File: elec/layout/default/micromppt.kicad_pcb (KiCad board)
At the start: 2 copper layers, 25.7 x 15.1 mm, 17 parts, among them U5 10µF ±20% 6.3V X5R

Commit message: fixed
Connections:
- C3 pad 1: hv-1 -> hv
- R1 pad 1: hv-1 -> hv
- R3 pad 1: hv -> hv-1
- R5 pad 2: hv-1 -> hv
- R6 pad 2: hv-1 -> hv
- U3 pad 1: hv -> hv-1
- U5 pad 1: hv -> hv-1
- U7 pad 1: hv-1 -> hv
- U8 pad 1: hv -> hv-1
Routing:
- net hv-1: track 18.5 -> 17.5 mm, vias 2 -> 0
- net hv: track 17.5 -> 18.5 mm, vias 0 -> 2
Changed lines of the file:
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@@
     (net 5 "cathode")
     (net 6 "VCTRL")
-    (net 7 "hv-1")
+    (net 7 "hv")
     (net 8 "gnd")
-    (net 9 "hv")
+    (net 9 "hv-1")
     (footprint "lib:SOT-23-6_L2.9-W1.6-P0.95-LS2.8-BR"
         (layer "F.Cu")
@@
             (size 0.57 0.54)
             (layers "F.Cu" "F.Mask" "F.Paste")
-            (net 7 "hv-1")
+            (net 7 "hv")
         )
         (pad "2" smd rect
@@
             (drill 0.900024)
             (layers "*.Cu" "*.Mask")
-            (net 9 "hv")
+            (net 9 "hv-1")
             (remove_unused_layers no)
         )
@@
             (size 0.8 0.9)
             (layers "F.Cu" "F.Mask" "F.Paste")
-            (net 9 "hv")
+            (net 9 "hv-1")
         )
         (pad "2" smd rect
@@
             (drill 0.900024)
             (layers "*.Cu" "*.Mask")
-            (net 7 "hv-1")
+            (net 7 "hv")
             (remove_unused_layers no)
         )
@@
             (size 0.57 0.54)
             (layers "F.Cu" "F.Mask" "F.Paste")
-            (net 7 "hv-1")
+            (net 7 "hv")
         )
         (embedded_fonts no)
@@
             (size 1.55 5.6)
             (layers "F.Cu" "F.Mask" "F.Paste")
-            (net 9 "hv")
+            (net 9 "hv-1")
             (pintype "stereo")
         )
@@
             (size 1.21 1.7)
             (layers "F.Cu" "F.Mask" "F.Paste")
-            (net 7 "hv-1")
+            (net 7 "hv")
         )
         (embedded_fonts no)
@@
             (size 0.8 0.9)
             (layers "F.Cu" "F.Mask" "F.Paste")
-            (net 7 "hv-1")
+            (net 7 "hv")
         )
         (pad "2" smd rect
@@
             (size 0.57 0.54)
             (layers "F.Cu" "F.Mask" "F.Paste")
-            (net 9 "hv")
+            (net 9 "hv-1")
         )
         (pad "2" smd rect

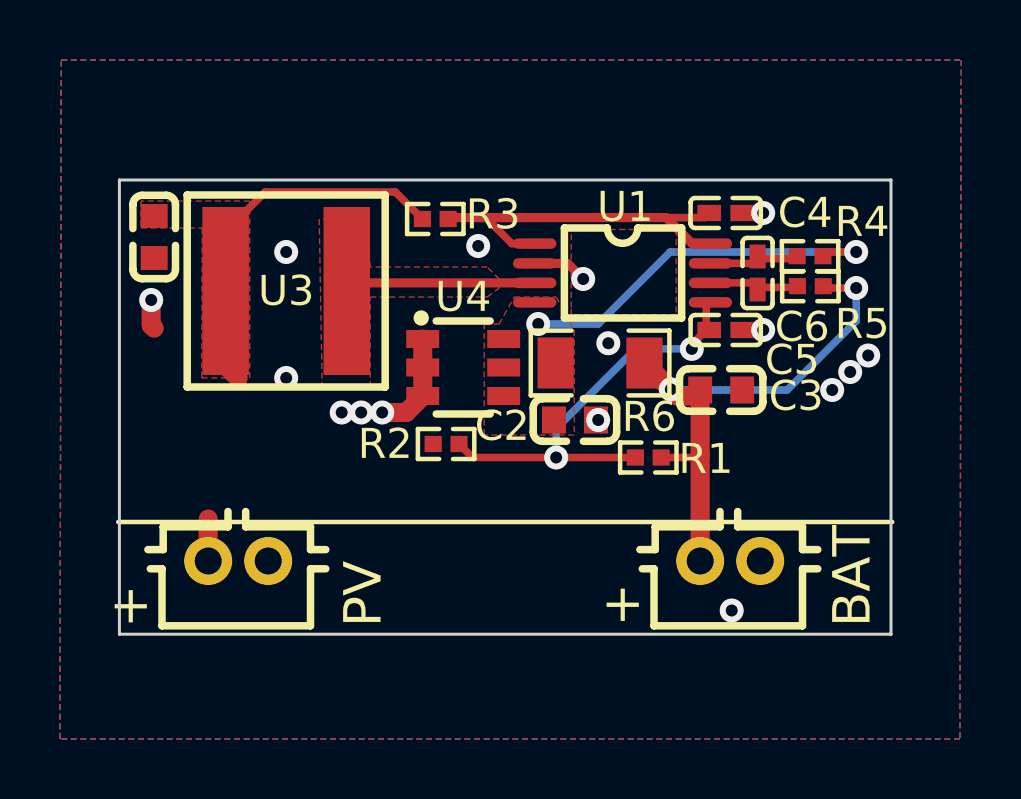
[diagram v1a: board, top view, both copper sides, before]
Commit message: ready for publishing on the ato repo
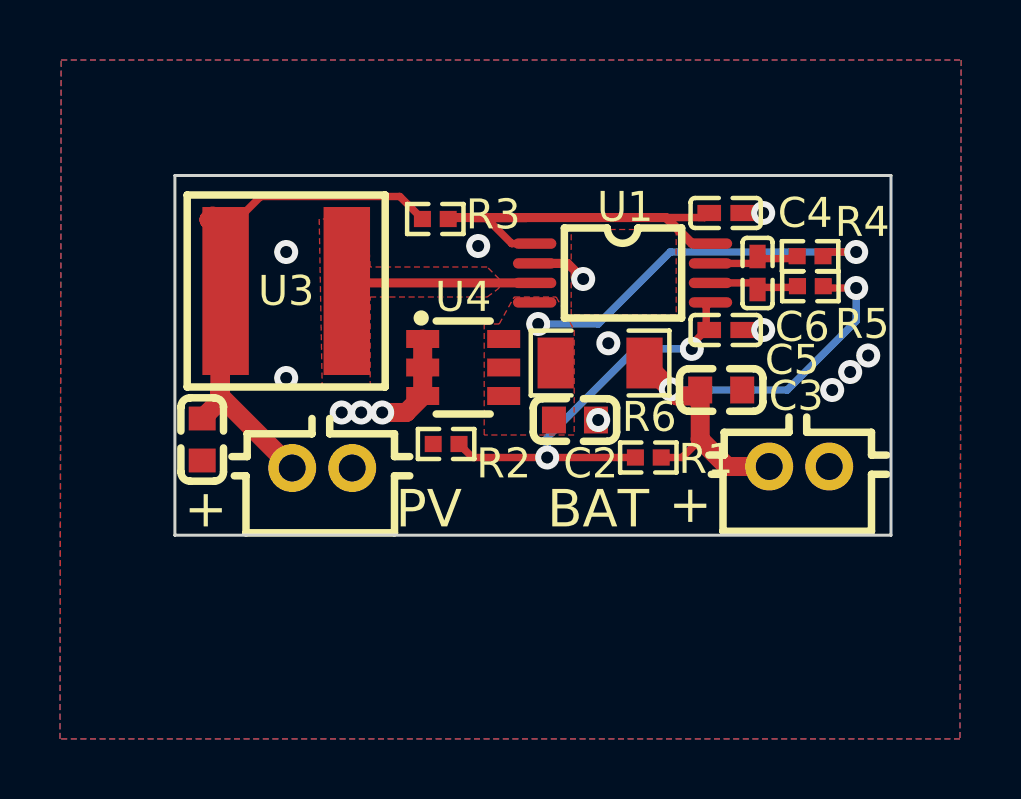
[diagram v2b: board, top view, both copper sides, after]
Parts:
- moved U5 6.94 mm to (69.2, 51.6)
- moved U8 4.18 mm to (73.2, 52.6)
- moved U7 3.90 mm to (89.1, 52.5)
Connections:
- net cathode renamed VOUT
- C3 pad 1: hv -> hv-1
- R1 pad 1: hv -> hv-1
- R3 pad 1: hv-1 -> hv
- R5 pad 2: hv -> hv-1
- R6 pad 2: hv -> hv-1
- U3 pad 1: hv-1 -> hv
- U5 pad 1: hv-1 -> hv
- U7 pad 1: hv -> hv-1
- U8 pad 1: hv-1 -> hv
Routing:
- net hv: track 18.5 -> 29.2 mm, vias 2 -> 0
- net gnd: track 6.29 -> 5.31 mm, vias 16 -> 14
- net hv-1: track 17.5 -> 17.4 mm, vias 0 -> 2
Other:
- board size 25.7 x 15.1 mm -> 23.9 x 12 mm
